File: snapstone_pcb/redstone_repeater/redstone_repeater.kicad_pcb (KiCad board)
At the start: 2 copper layers, 101.1 x 49 mm, 17 parts, among them SW1 SW_Push, SW2 SW_Push, SW3 SW_Push, SW4 SW_Push, U1 MOUDLE-SEEEDUINO-XIAO, U2 Current Sensor

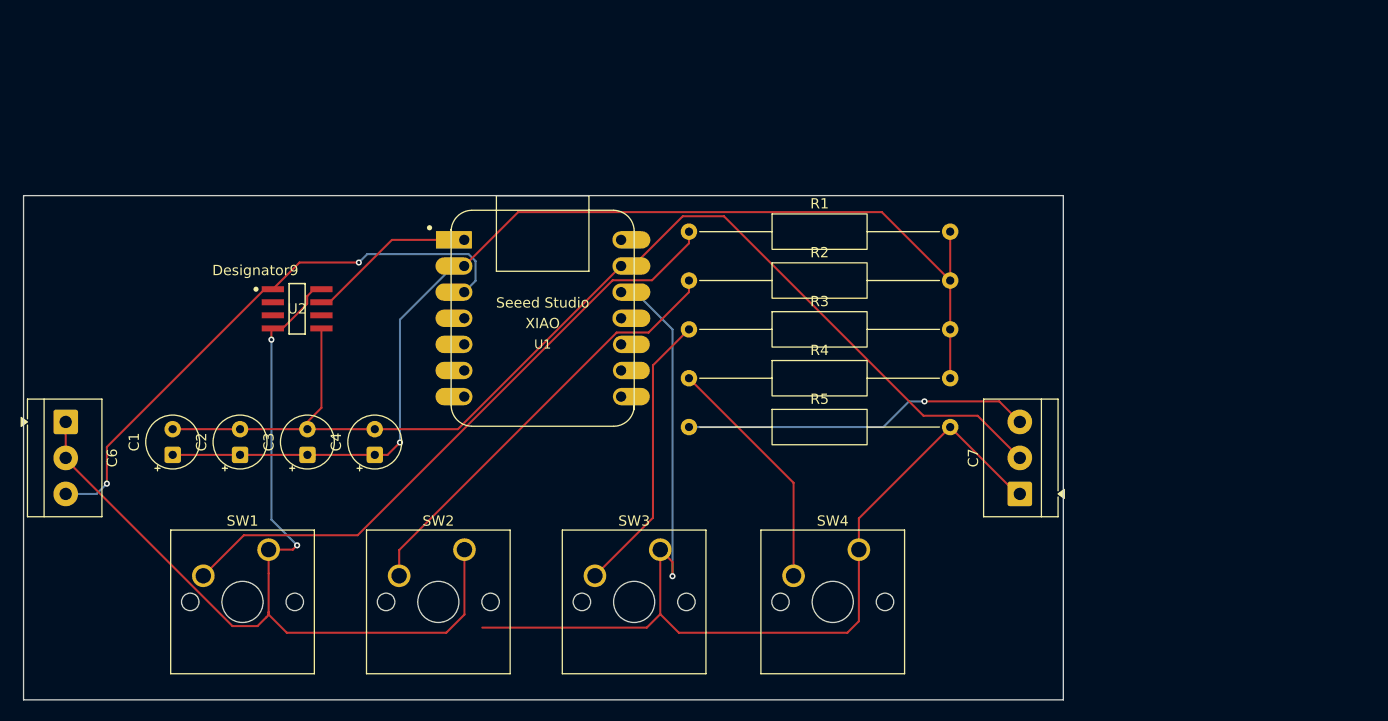
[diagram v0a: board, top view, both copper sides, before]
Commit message: did a bunch of stuff (something something Redstone Repeater PCB Changes)
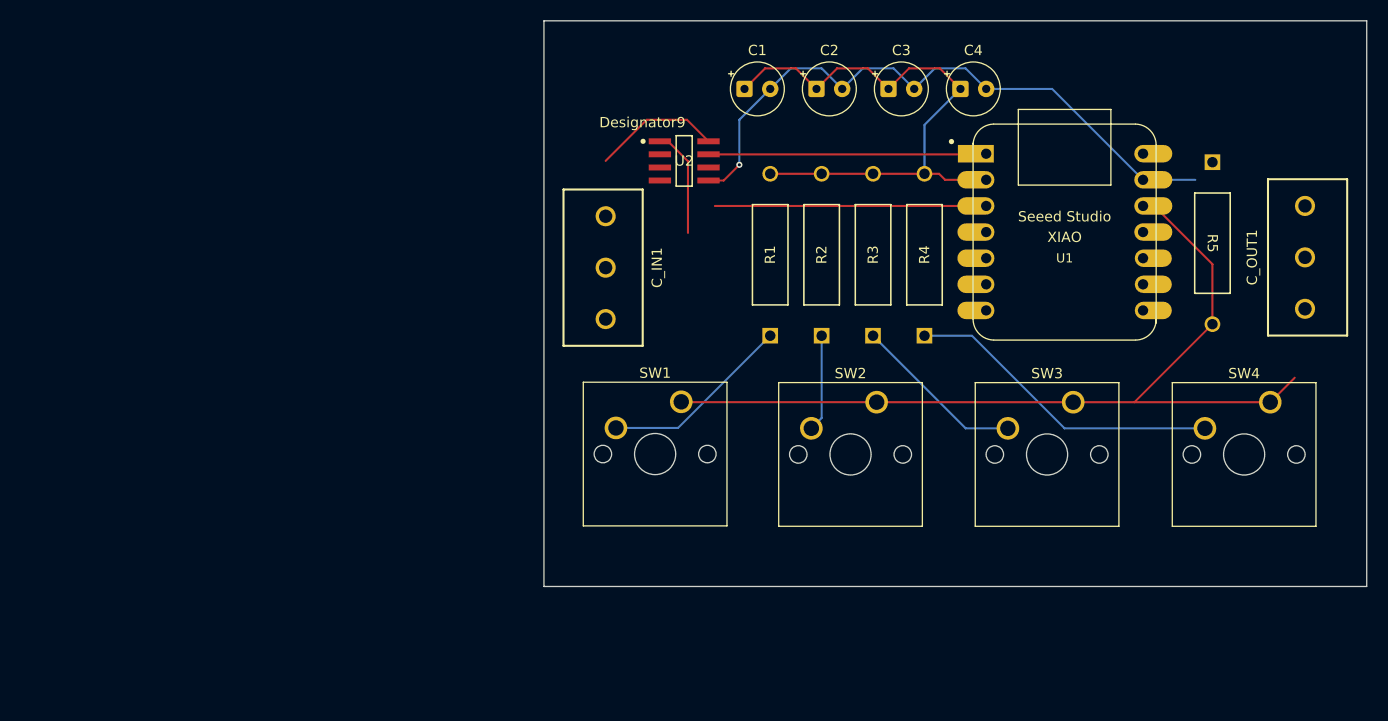
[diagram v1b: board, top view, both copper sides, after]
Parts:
- removed C6, C7: ~, TerminalBlock_4Ucon:TerminalBlock_4Ucon_1x03_P3.50mm_Horizontal
- added C_IN1: ~, 691137710003_Board_To_Wire:691137710003_Board_To_Wire, F.Cu at (116.0, 109.0)
- added C_OUT1: ~, 691137710003_Board_To_Wire:691137710003_Board_To_Wire, F.Cu at (184.0, 108.0)
- R1, R2, R3, R4, R5: footprint Resistor_THT:R_Axial_DIN0309_L9.0mm_D3.2mm_P25.40mm_Horizontal -> CF12JT150R_Resistor_150:STA_CF12_STP
- moved C4 67.2 mm to (150.5, 91.6), turned to 0 degrees
- moved C3 66.8 mm to (143.5, 91.6), turned to 0 degrees
- moved C2 66.4 mm to (136.5, 91.6), turned to 0 degrees
- moved C1 66.0 mm to (129.5, 91.6), turned to 0 degrees
- moved R5 57.0 mm to (175.0, 98.7), turned to -90 degrees
- moved U1 51.4 mm to (160.6, 105.5)
- moved SW3 42.6 mm to (161.5, 122.1)
- moved SW1 42.6 mm to (123.3, 122.0)
- moved SW2 42.6 mm to (142.3, 122.1)
- moved SW4 42.5 mm to (180.6, 122.1)
- moved U2 40.3 mm to (123.6, 98.6)
- moved R4 23.3 mm to (147.0, 115.6), turned to 90 degrees
- moved R3 17.9 mm to (142.0, 115.6), turned to 90 degrees
- moved R2 14.0 mm to (137.0, 115.6), turned to 90 degrees
- moved R1 12.8 mm to (132.0, 115.6), turned to 90 degrees
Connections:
- U2 pad 4: VCC -> unconnected-(U2-IN--Pad4)
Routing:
- net VCC: track 206.0 -> 98.9 mm, vias 3 -> 0
- net TDD: track 109.4 -> 56.9 mm, vias 1 -> 0
- net GND: track 111.0 -> 62.2 mm, vias 0 -> 1
- net Net-(R1-Pad1): track 61.7 -> 18.7 mm
- net Net-(C_OUT1-DAT): track 34.0 -> 0.00 mm, vias 1 -> 0
- net Net-(R2-Pad1): track 42.2 -> 9.41 mm
- net DAT: track 55.3 -> 36.9 mm, vias 2 -> 0
- net Net-(R3-Pad1): track 27.7 -> 16.8 mm
- net AOUT: track 16.4 -> 27.0 mm
- net Net-(R4-Pad1): track 23.4 -> 31.0 mm
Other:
- board size 101.1 x 49 mm -> 80 x 55 mm
